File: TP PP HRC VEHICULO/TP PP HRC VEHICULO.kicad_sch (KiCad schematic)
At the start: 48 parts, among them J1 Screw_Terminal_01x02, J2 Screw_Terminal_01x03, J3 Screw_Terminal_01x03, J4 USB_B, J5 Conn_01x02_Pin, J6 Conn_01x04_Pin, J7 Conn_01x01_Pin, J8 Conn_01x01_Pin, K1 Relay_SPDT, K2 Relay_SPDT, Q1 S8050, Q2 S8050, Q3 S8050, SW1 SW_DPST_x2, SW2 SW_Push, SW3 SW_Push, U1 ESP32-Devkit-V1, U2 LM317_TO-220

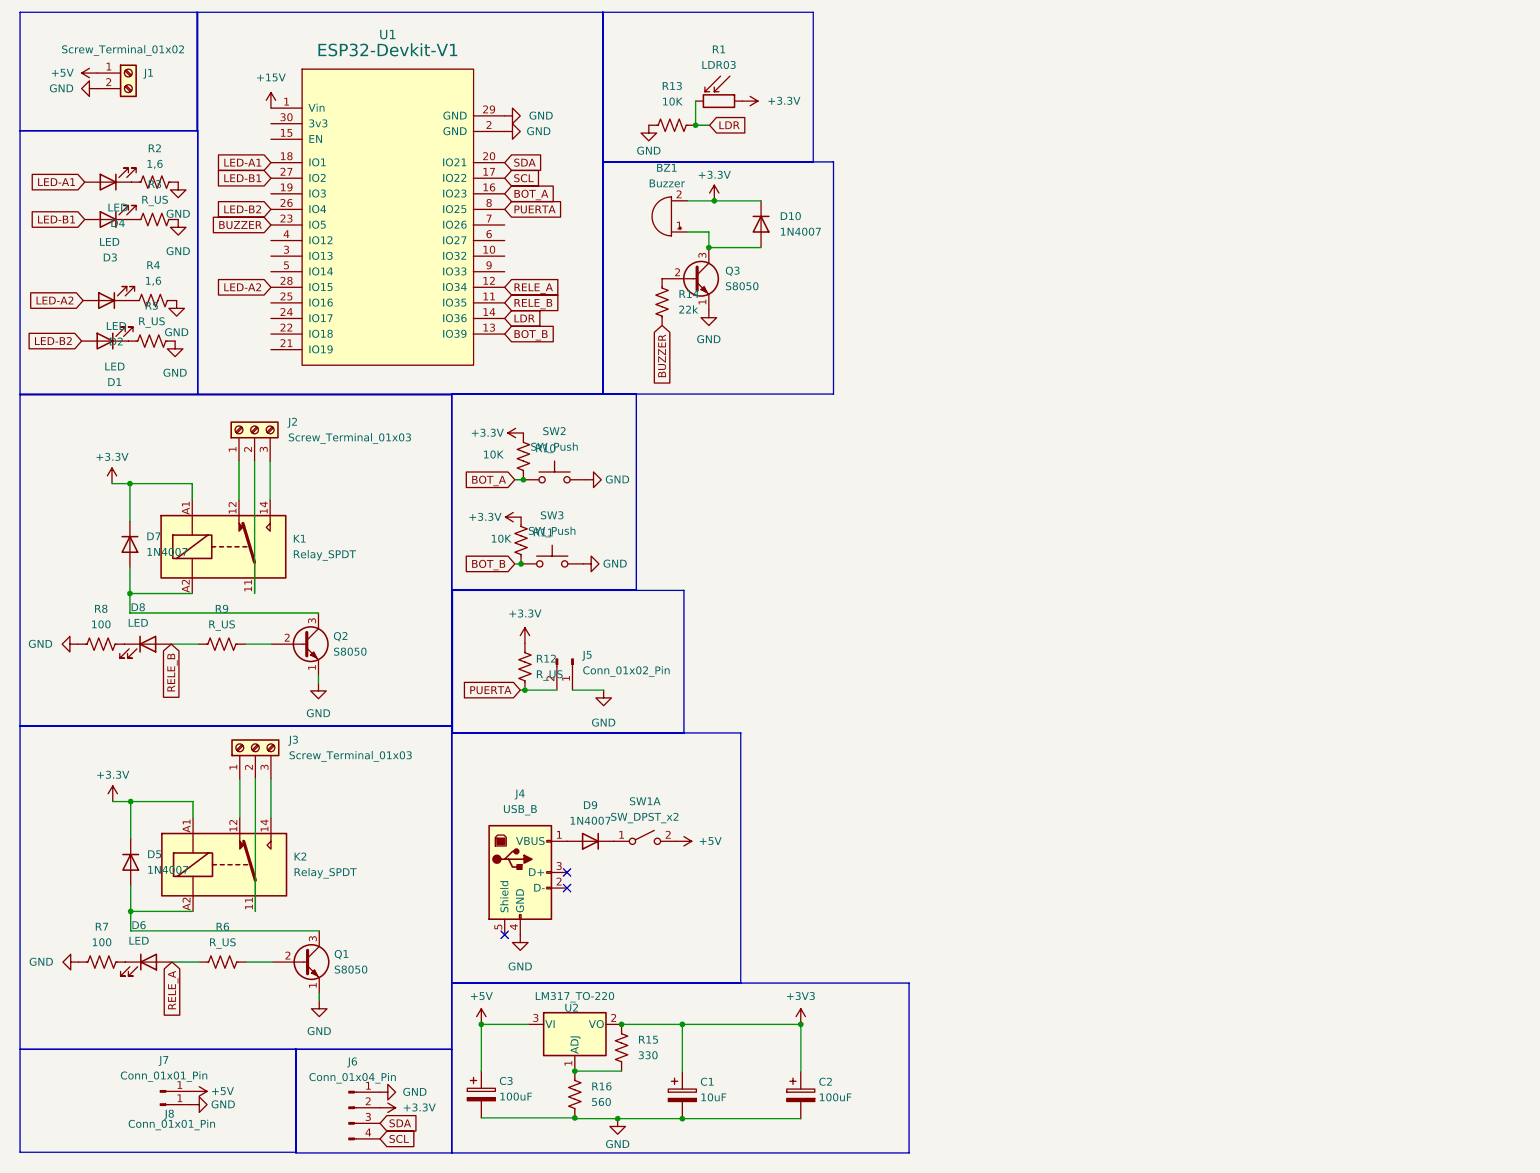
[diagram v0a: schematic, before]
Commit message: placa
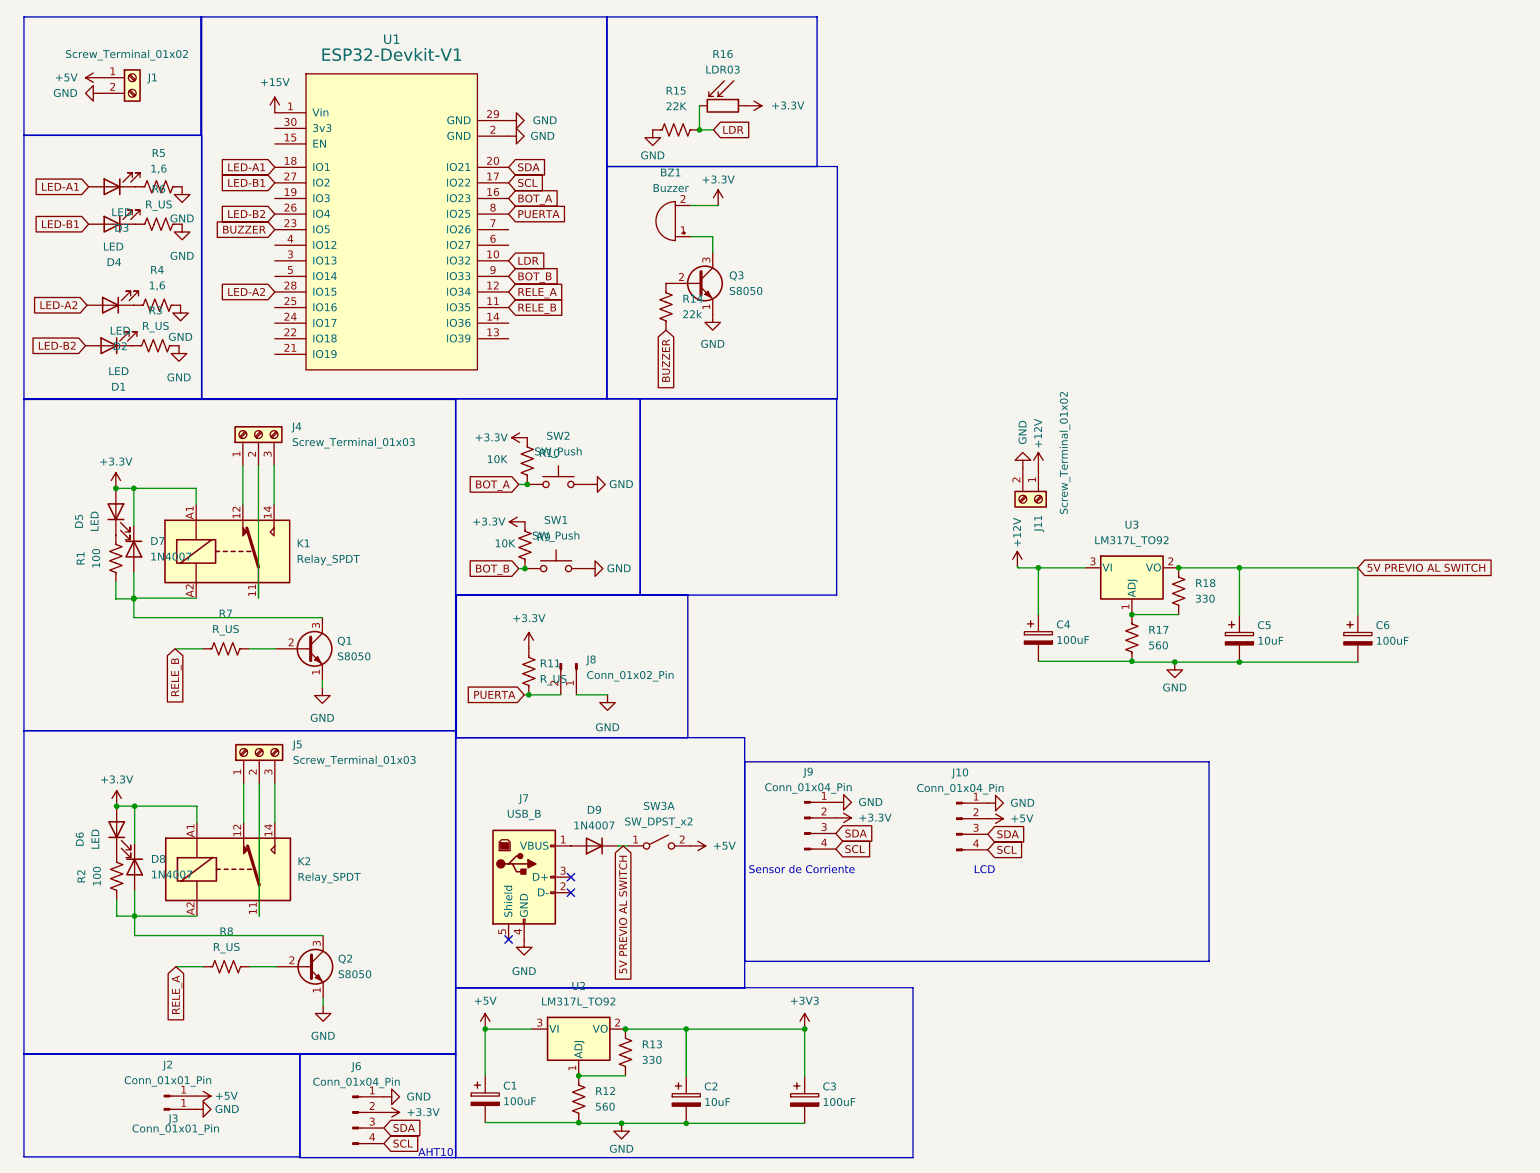
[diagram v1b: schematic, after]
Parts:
- removed D10, D5: 1N4007, Diode_THT:D_DO-41_SOD81_P10.16mm_Horizontal, symbol Diode:1N4007
- removed D8: LED, LED_THT:LED_D5.0mm, symbol Device:LED
- removed J2, J3: Screw_Terminal_01x03, TerminalBlock:TerminalBlock_bornier-3_P5.08mm, symbol Connector:Screw_Terminal_01x03
- removed J4: USB_B, Connector_USB:USB_B_OST_USB-B1HSxx_Horizontal, symbol Connector:USB_B
- removed J5: Conn_01x02_Pin, Connector_Molex:Molex_KK-254_AE-6410-02A_1x02_P2.54mm_Vertical, symbol Connector:Conn_01x02_Pin
- removed J7, J8: Conn_01x01_Pin, Connector_Molex:Molex_KK-254_AE-6410-04A_1x04_P2.54mm_Vertical, symbol Connector:Conn_01x01_Pin
- removed R1: LDR03, Connector_Molex:Molex_KK-254_AE-6410-02A_1x02_P2.54mm_Vertical, symbol Sensor_Optical:LDR03
- removed R16: 560, Resistor_THT:R_Axial_DIN0207_L6.3mm_D2.5mm_P10.16mm_Horizontal, symbol Device:R_US
- removed SW1: SW_DPST_x2, TerminalBlock:TerminalBlock_bornier-2_P5.08mm, symbol Switch:SW_DPST_x2
- removed SW3: SW_Push, Connector_Molex:Molex_CLIK-Mate_502382-0270_1x02-1MP_P1.25mm_Vertical, symbol Switch:SW_Push
- removed U2: LM317_TO-220, Package_TO_SOT_THT:TO-220-3_Vertical, symbol Regulator_Linear:LM317_TO-220
- added C4: 100uF, Capacitor_THT:CP_Radial_D10.0mm_P3.50mm, symbol Device:C_Polarized
- added C5: 10uF, Capacitor_THT:CP_Radial_D5.0mm_P2.50mm, symbol Device:C_Polarized
- added C6: 100uF, Capacitor_THT:C_Disc_D7.5mm_W4.4mm_P5.00mm, symbol Device:C_Polarized
- added D5: LED, LED_THT:LED_D5.0mm, symbol Device:LED
- added D8: 1N4007, Diode_THT:D_DO-41_SOD81_P10.16mm_Horizontal, symbol Diode:1N4007
- added J10, J9: Conn_01x04_Pin, Connector_Molex:Molex_KK-254_AE-6410-04A_1x04_P2.54mm_Vertical, symbol Connector:Conn_01x04_Pin
- added J11: Screw_Terminal_01x02, TerminalBlock:TerminalBlock_bornier-2_P5.08mm, symbol Connector:Screw_Terminal_01x02
- added J2, J3: Conn_01x01_Pin, Connector_Molex:Molex_KK-254_AE-6410-04A_1x04_P2.54mm_Vertical, symbol Connector:Conn_01x01_Pin
- added J4, J5: Screw_Terminal_01x03, TerminalBlock:TerminalBlock_bornier-3_P5.08mm, symbol Connector:Screw_Terminal_01x03
- added J7: USB_B, Connector_USB:USB_B_OST_USB-B1HSxx_Horizontal, symbol Connector:USB_B
- added J8: Conn_01x02_Pin, Connector_Molex:Molex_KK-254_AE-6410-02A_1x02_P2.54mm_Vertical, symbol Connector:Conn_01x02_Pin
- added R1: 100, Resistor_THT:R_Axial_DIN0207_L6.3mm_D2.5mm_P10.16mm_Horizontal, symbol Device:R_US
- added R16: LDR03, Connector_Molex:Molex_KK-254_AE-6410-02A_1x02_P2.54mm_Vertical, symbol Sensor_Optical:LDR03
- added R17: 560, Resistor_THT:R_Axial_DIN0207_L6.3mm_D2.5mm_P10.16mm_Horizontal, symbol Device:R_US
- added R18: 330, Resistor_THT:R_Axial_DIN0207_L6.3mm_D2.5mm_P10.16mm_Horizontal, symbol Device:R_US
- added SW1: SW_Push, Connector_Molex:Molex_KK-254_AE-6410-02A_1x02_P2.54mm_Vertical, symbol Switch:SW_Push
- added SW3: SW_DPST_x2, TerminalBlock:TerminalBlock_bornier-2_P5.08mm, symbol Switch:SW_DPST_x2
- added U2, U3: LM317L_TO92, Package_TO_SOT_THT:TO-92_Inline, symbol Regulator_Linear:LM317L_TO92
- C1: value 10uF -> 100uF; footprint Capacitor_THT:CP_Radial_D5.0mm_P2.50mm -> Capacitor_THT:CP_Radial_D10.0mm_P3.50mm
- C2: value 100uF -> 10uF; footprint Capacitor_THT:C_Disc_D7.5mm_W4.4mm_P5.00mm -> Capacitor_THT:CP_Radial_D5.0mm_P2.50mm
- C3: footprint Capacitor_THT:CP_Radial_D10.0mm_P3.50mm -> Capacitor_THT:C_Disc_D7.5mm_W4.4mm_P5.00mm
- J6: footprint (none) -> Connector_Molex:Molex_KK-254_AE-6410-04A_1x04_P2.54mm_Vertical
- R11: value 10K -> R_US
- R12: value R_US -> 560
- R13: value 10K -> 330
- R15: value 330 -> 22K
- R2: value 1,6 -> 100
- R5: value R_US -> 1,6
- R7, R8: value 100 -> R_US
- R9: value R_US -> 10K
- SW2: footprint Button_Switch_THT:SW_PUSH_6mm_H4.3mm -> Connector_Molex:Molex_KK-254_AE-6410-02A_1x02_P2.54mm_Vertical
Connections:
- net +3.3V: now also D6.2 (A), R11.1, R9.2, D5.2 (A), D8.1 (K), J9.2 (Pin_2), R16.1; no longer R11.2, R12.1
- net +3V3: now also C3.1, R13.1, U2.2 (VO); no longer C1.1, R15.1
- net +5V: now also C1.1, J10.2 (Pin_2), J2.1 (Pin_1), SW3.2 (B), U2.3 (VI); no longer C3.1
- net BOT_B: now also R9.1, U1.9 (IO33), SW1.1; no longer R11.1, U1.13 (IO39)
- net GND: now also R12.2, R15.1, R6.2, C4.2, C5.2, C6.2, J10.1 (Pin_1), J11.2 (Pin_2), J3.1 (Pin_1), J7.4 (GND), J8.1 (Pin_1), J9.1 (Pin_1), R17.2, SW1.2; no longer R13.1, R2.2, R7.1, R8.1
- net LDR: now also R15.2, U1.10 (IO32), R16.2; no longer R13.2, U1.14 (IO36)
- net LED-A1: now also D3.2 (A); no longer D4.2 (A)
- net LED-B1: now also D4.2 (A); no longer D3.2 (A)
- net PUERTA: now also R11.2, J8.2 (Pin_2); no longer R12.2
- net RELE_A: now also R8.1; no longer D6.2 (A), R6.1
- net RELE_B: now also R7.1; no longer R9.1
- net SCL: now also J10.4 (Pin_4), J9.4 (Pin_4)
- net SDA: now also J10.3 (Pin_3), J9.3 (Pin_3)
- net at D4.1 (K): now also R6.1; no longer R2.1
- net at D7.2 (A), K1.A2: now also Q1.3 (C), R1.1; no longer Q2.3 (C)
- net at D1.1 (K): now also R3.1; no longer R5.1
- net at D6.1 (K): now also R2.2; no longer R7.2
- net at Q2.2 (B): now also R8.2; no longer R9.2
- net 5V PREVIO AL SWITCH: now reaches D9.1 (K)
- net 5V PREVIO AL SWITCH: now also C5.1, C6.1, R18.1, SW3.1 (A), U3.2 (VO)
- net at D9.2 (A): now also J7.1 (VBUS)
- net at D3.1 (K): now also R5.1; no longer R3.1
- net at K2.11: now also J5.2 (Pin_2)
- net at K2.12: now also J5.1 (Pin_1)
- net at K2.14: now also J5.3 (Pin_3)
- net at K2.A2: now also Q2.3 (C), R2.1, D8.2 (A); no longer Q1.3 (C)
- net at Q1.2 (B): now also R7.2; no longer R6.2
- net at K1.11: now also J4.2 (Pin_2)
- net at K1.12: now also J4.1 (Pin_1)
- net at K1.14: now also J4.3 (Pin_3)
- new net: D5.1 (K), R1.2
- new net: R12.1, R13.2, U2.1 (ADJ)
- new net: R17.1, R18.2, U3.1 (ADJ)
- new net +12V: C4.1, J11.1 (Pin_1), U3.3 (VI)
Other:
- note added: "AHT10"
- note added: "LCD"
- note added: "Sensor de Corriente"

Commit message: placa actualizada
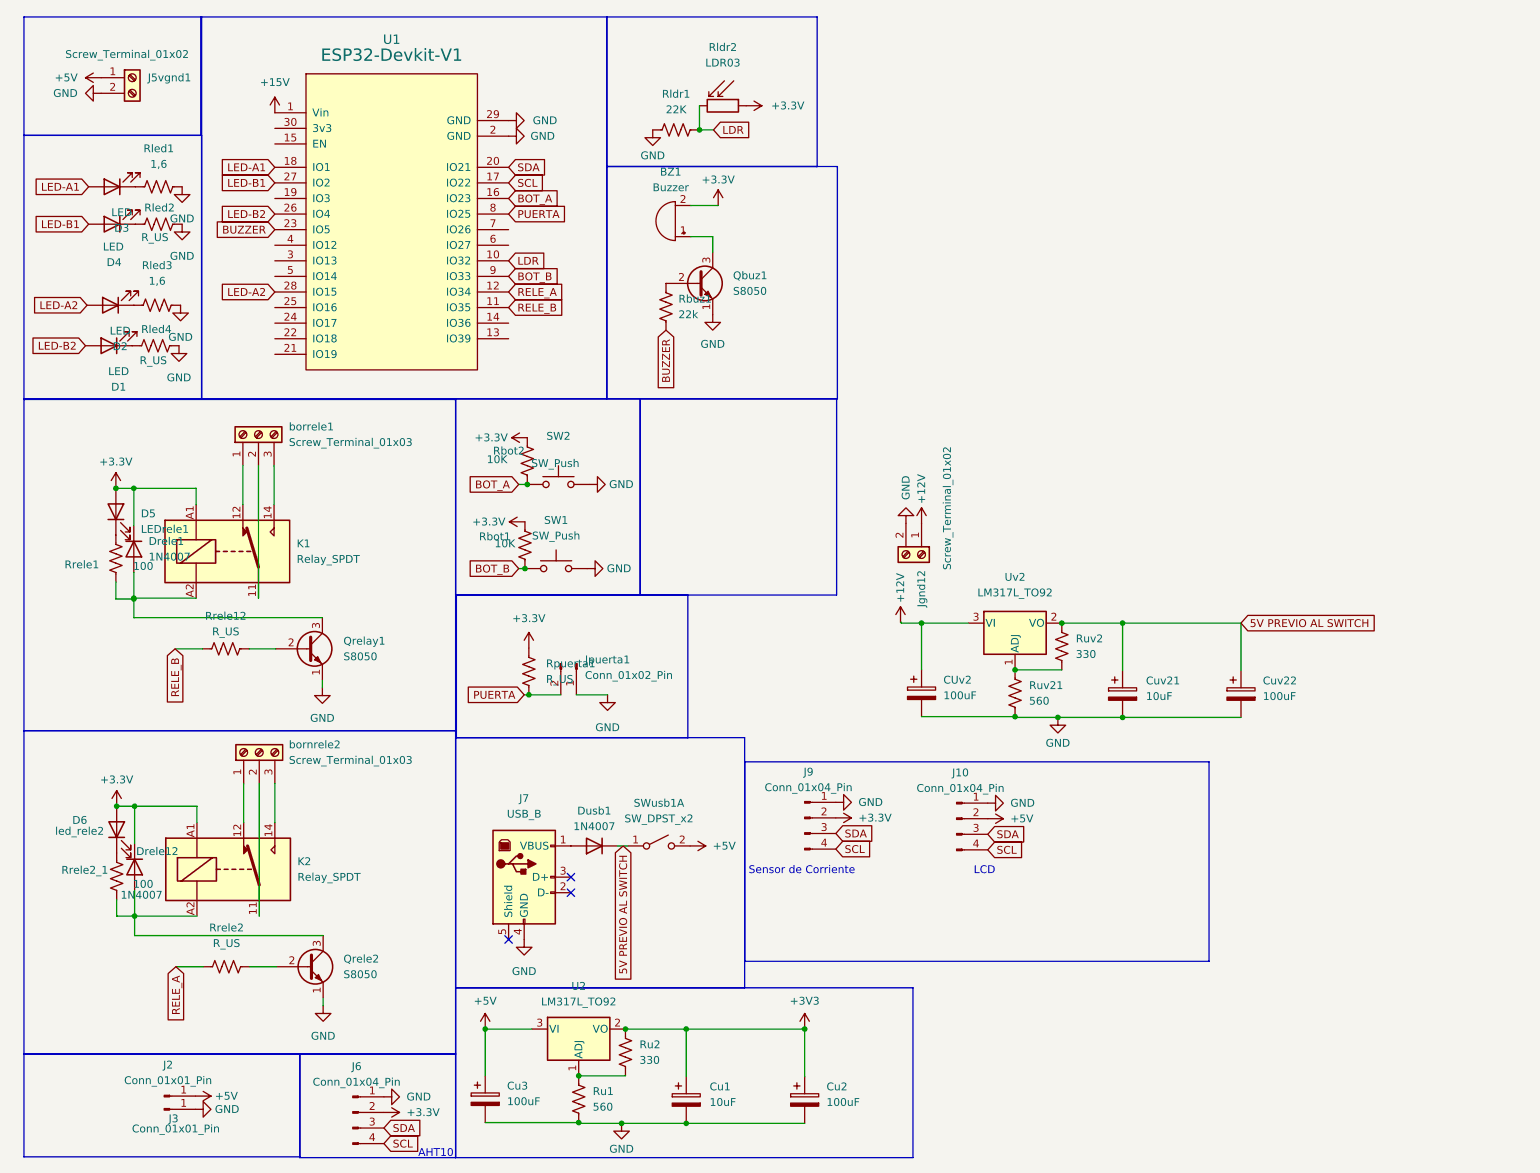
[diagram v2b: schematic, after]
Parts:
- D5: value LED -> LEDrele1
- D6: value LED -> led_rele2
- renumbered C4 to CUv2, C2 to Cu1, C3 to Cu2, C1 to Cu3, C5 to Cuv21, C6 to Cuv22, D7 to Drele1, D8 to Drele12, D9 to Dusb1, J1 to J5vgnd1, J11 to Jgnd12, J8 to Jpuerta1, Q3 to Qbuz1, Q1 to Qrelay1, Q2 to Qrele2, R9 to Rbot1, R10 to Rbot2, R14 to Rbuz1, R15 to Rldr1, R16 to Rldr2, R5 to Rled1, R6 to Rled2, R4 to Rled3, R3 to Rled4, R11 to Rpuerta1, R1 to Rrele1, R7 to Rrele12, R8 to Rrele2, R2 to Rrele2_1, R12 to Ru1, R13 to Ru2, R18 to Ruv2, R17 to Ruv21, SW3 to SWusb1, U3 to Uv2, J5 to bornrele2, J4 to borrele1
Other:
- moved on the sheet: CUv2, Cuv21, Cuv22, Jgnd12, Ruv2, Ruv21, Uv2
